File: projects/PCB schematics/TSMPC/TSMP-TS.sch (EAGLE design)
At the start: 23 parts, among them J1 2P_1-770166-0, J2 2P_1-770166-0, J3 2P_1-770166-0

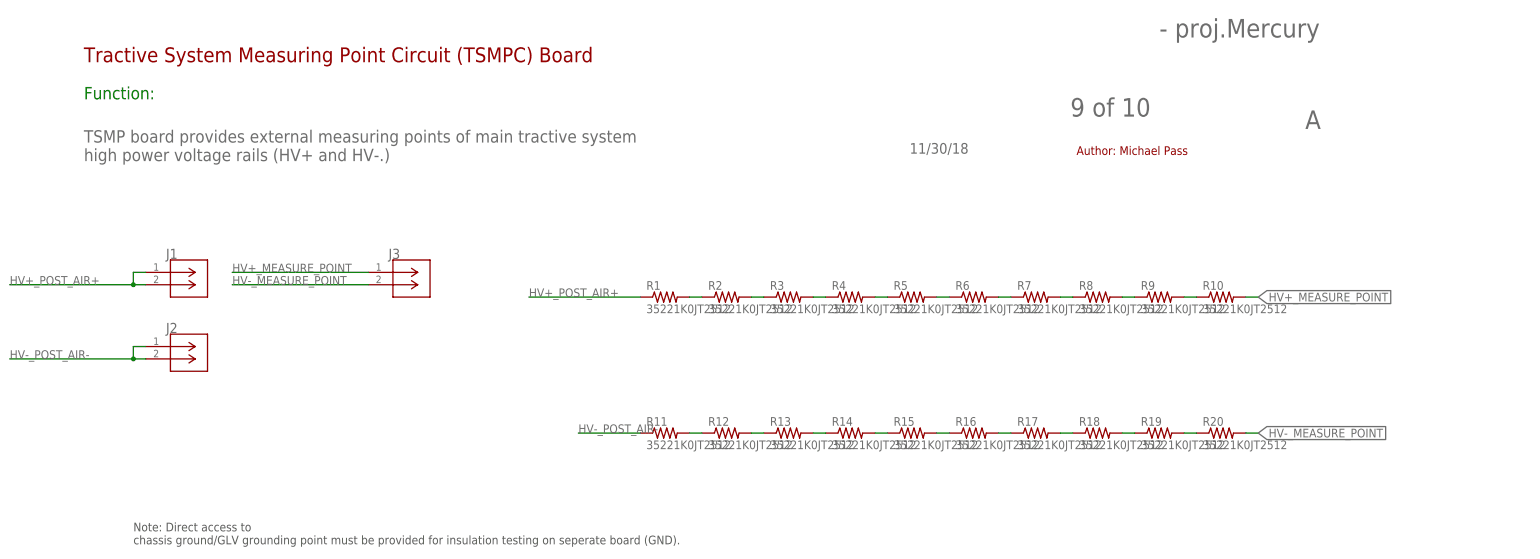
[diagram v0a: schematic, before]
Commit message: PROJ - Final pre-purchase revisions (4 boards still in progress.)
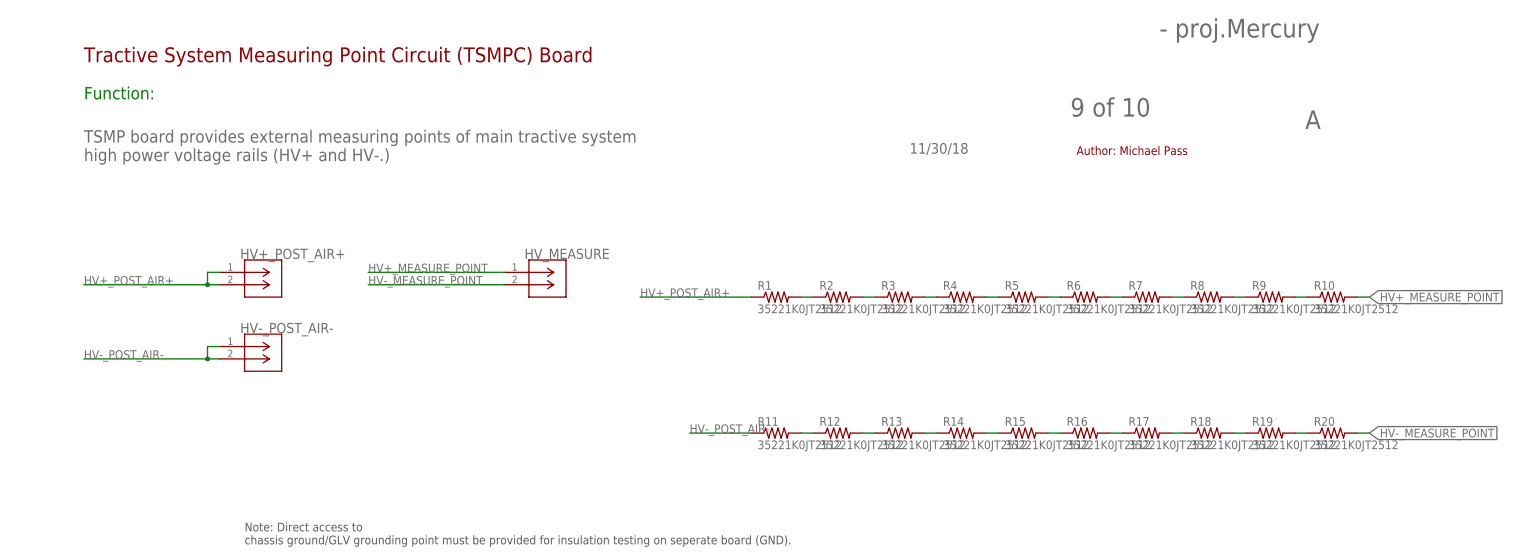
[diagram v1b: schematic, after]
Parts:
- removed J1, J2, J3: 2P_1-770166-0, con-MATE-N-LOK:2P_1-770166-0
- added HV+_POST_AIR+, HV-_POST_AIR-, HV_MEASURE: 2P_1-770166-0, con-MATE-N-LOK:2P_1-770166-0
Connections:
- net HV+_MEASURE_POINT: now also HV_MEASURE.1; no longer J3.1
- net HV+_POST_AIR+: now also HV+_POST_AIR+.1, HV+_POST_AIR+.2; no longer J1.1, J1.2
- net HV-_MEASURE_POINT: now also HV_MEASURE.2; no longer J3.2
- net HV-_POST_AIR-: now also HV-_POST_AIR-.1, HV-_POST_AIR-.2; no longer J2.1, J2.2
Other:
- moved on the sheet: R1, R10, R11, R12, R13, R14, R15, R16, R17, R18, R19, R2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
